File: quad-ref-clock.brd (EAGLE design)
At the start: 48 x 48 mm, 29 parts, among them U1 LMK00804B, U2 ADP150, U3 ADP150, X1 SMA, X2 SMA, X3 SMA, X4 SMA

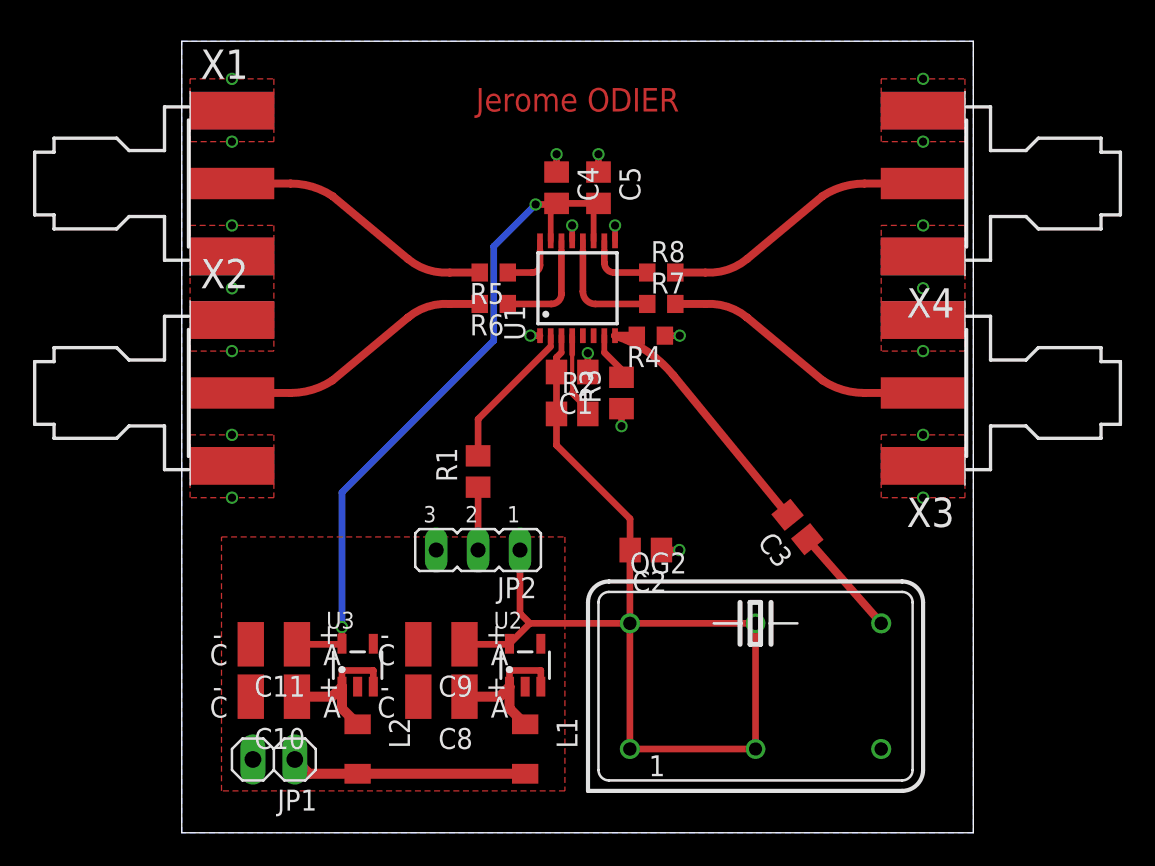
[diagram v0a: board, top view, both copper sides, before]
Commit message: update
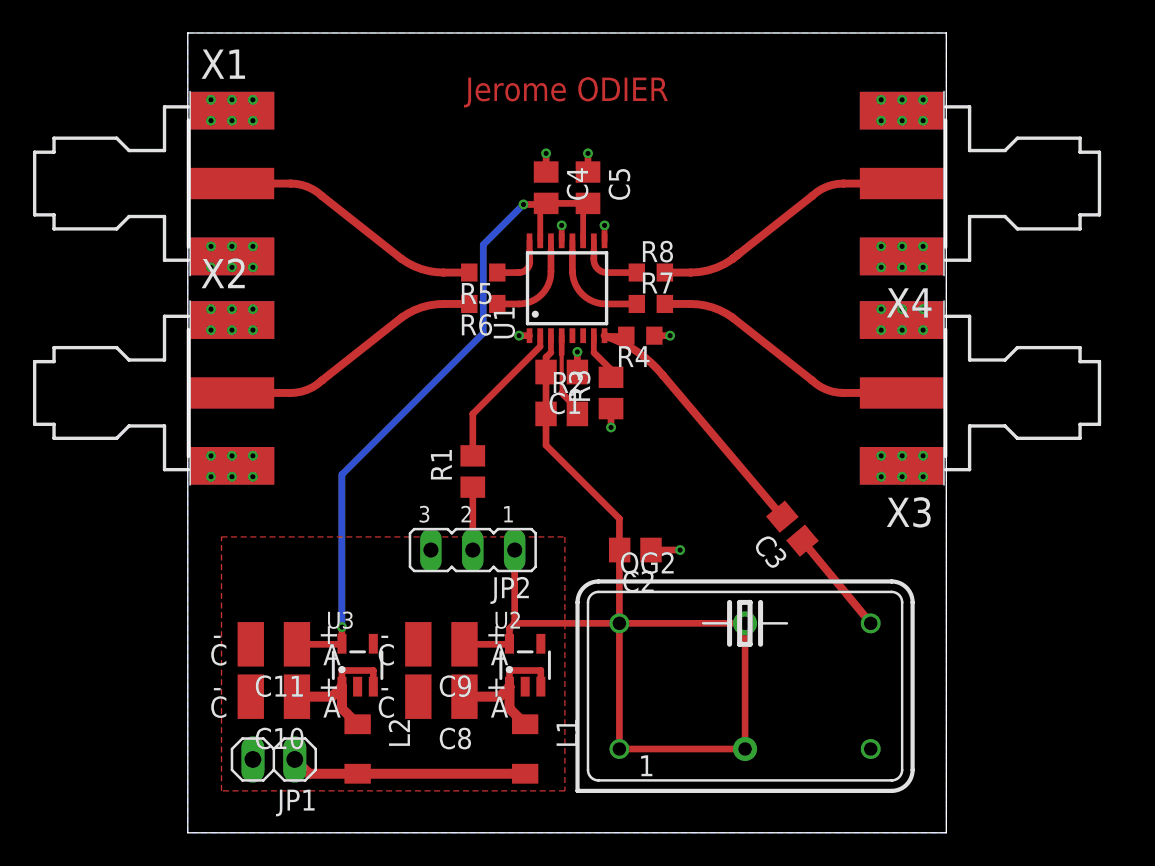
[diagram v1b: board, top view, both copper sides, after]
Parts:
- moved X3 1.27 mm to (45.7, 26.7)
- moved X4 1.27 mm to (45.7, 39.4)
- moved C1 0.64 mm to (22.5, 27.9)
- moved C2 0.64 mm to (27.0, 17.1)
- moved C4 0.64 mm to (21.6, 39.1)
- moved C5 0.64 mm to (24.1, 39.1)
- moved R2 0.64 mm to (22.5, 25.4)
- moved R4 0.64 mm to (27.3, 30.1)
- moved U1 0.64 mm to (22.9, 33.0)
- moved QG2 0.63 mm to (33.7, 8.89)
- moved R3 0.63 mm to (25.5, 26.7)
- moved R5 0.63 mm to (17.8, 34.0)
- moved R6 0.63 mm to (17.8, 32.1)
- moved R7 0.63 mm to (27.9, 32.1)
- moved R8 0.63 mm to (27.9, 34.0)
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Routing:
- net GND: track 8.81 -> 9.85 mm, vias 23 -> 57
- net N$2: track 6.72 -> 5.94 mm
- net N$3: track 7.29 -> 6.56 mm
- net N$11: track 16.6 -> 16.0 mm
- net N$10: track 16.6 -> 16.0 mm
- net N$12: track 16.6 -> 16.0 mm
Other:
- board size 48 x 48 mm -> 46 x 48.5 mm
